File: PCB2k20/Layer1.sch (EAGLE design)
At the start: 279 parts, among them J1 XT30PB-F, J10 14AWG, J11 14AWG, J13 14AWG, J14 14AWG, J15 14AWG, J16 14AWG, J17 14AWG, J18 14AWG, J19 14AWG, J20 14AWG, J3 14AWG, J4 14AWG, J5 14AWG, J6 14AWG, J7 14AWG, J8 14AWG, J9 14AWG, Q1M1 AOD482, Q1M2 AOD482, Q1M3 AOD482, Q1M4 AOD482, U1M1 VNH5019, U1M2 VNH5019, U1M3 VNH5019, U1M4 VNH5019, X1 BM10B-SRSS-TB

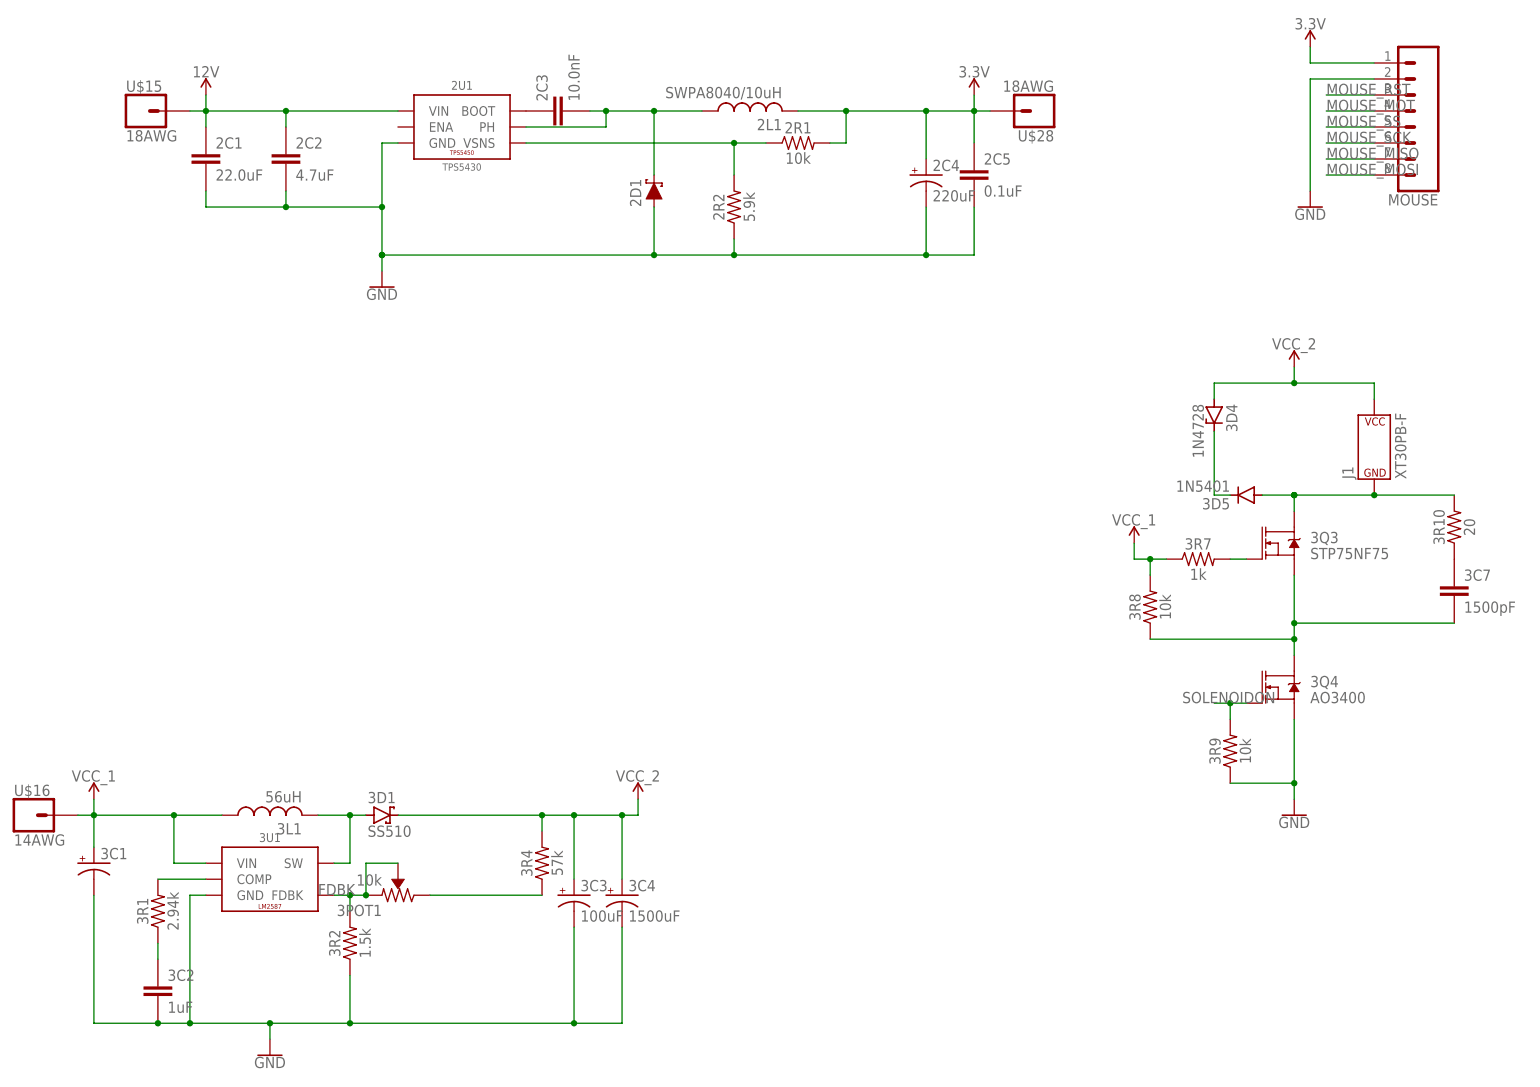
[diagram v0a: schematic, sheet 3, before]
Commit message: add gerbers, please everything turn out well!
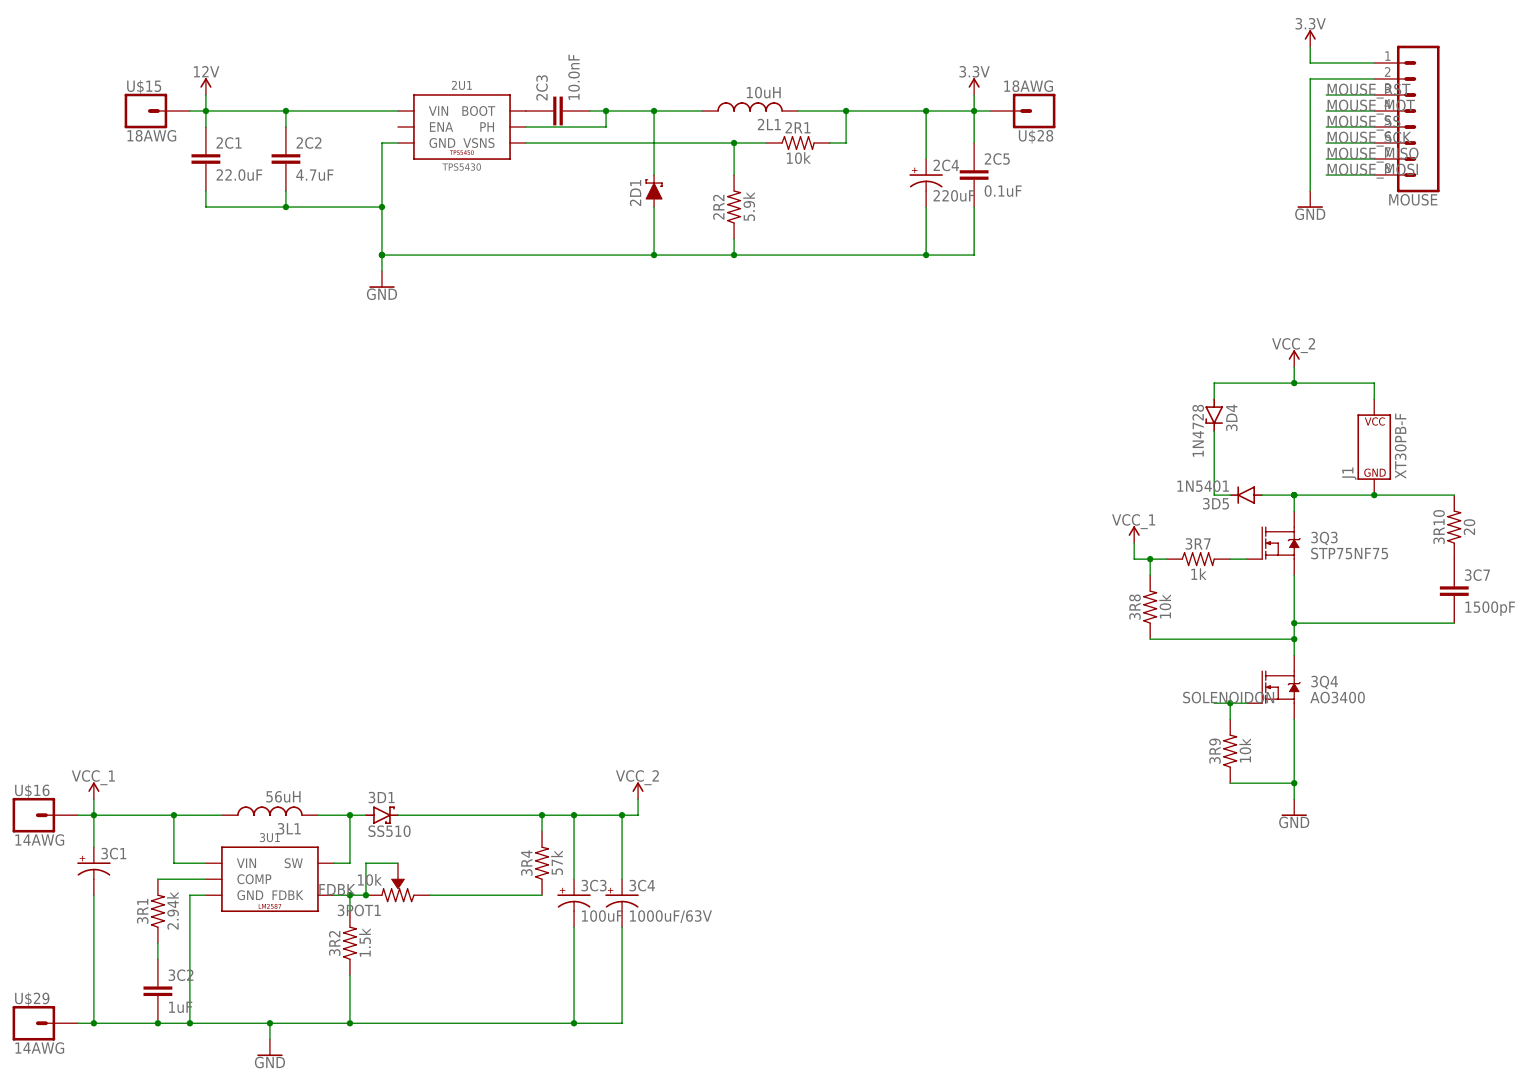
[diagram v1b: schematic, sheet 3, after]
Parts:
- added J21, U$29: 14AWG, JH:14AWG
- 2L1: value SWPA8040/10uH -> 10uH
- 3C4: value 1500uF -> 1000uF/63V
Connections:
- net GND: now also J21.1, U$29.1
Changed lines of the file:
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@@
 <part name="2C3" library="JH" library_urn="urn:adsk.eagle:library:6027132" deviceset="CAPACITOR" device="0603" package3d_urn="urn:adsk.eagle:package:15441226/3" value="10.0nF"/>
 <part name="2D1" library="SparkFun-DiscreteSemi" library_urn="urn:adsk.eagle:library:514" deviceset="DIODE-SCHOTTKY" device="-B340A" package3d_urn="urn:adsk.eagle:package:38443/1" value="3A/40V/500mV"/>
-<part name="2L1" library="JH" library_urn="urn:adsk.eagle:library:6027132" deviceset="INDUCTOR" device="SWPA8040" package3d_urn="urn:adsk.eagle:package:15402033/4" value="SWPA8040/10uH"/>
+<part name="2L1" library="JH" library_urn="urn:adsk.eagle:library:6027132" deviceset="INDUCTOR" device="SWPA8040" package3d_urn="urn:adsk.eagle:package:15402033/4" value="10uH"/>
 <part name="2R1" library="JH" library_urn="urn:adsk.eagle:library:6027132" deviceset="RESISTOR" device="0603" package3d_urn="urn:adsk.eagle:package:15441228/3" value="10k"/>
 <part name="2C4" library="rcl" library_urn="urn:adsk.eagle:library:334" deviceset="CPOL-US" device="D/7343-31R" package3d_urn="urn:adsk.eagle:package:23417/2" value="220uF"/>
@@
 <part name="SUPPLY25" library="SparkFun-PowerSymbols" library_urn="urn:adsk.eagle:library:530" deviceset="12V" device=""/>
 <part name="SUPPLY26" library="SparkFun-PowerSymbols" library_urn="urn:adsk.eagle:library:530" deviceset="3.3V" device=""/>
-<part name="CONN_M1" library="JH" library_urn="urn:adsk.eagle:library:6027132" deviceset="XT30" device="PB-F" package3d_urn="urn:adsk.eagle:package:15925142/4"/>
+<part name="CONN_M1" library="JH" library_urn="urn:adsk.eagle:library:6027132" deviceset="XT30" device="PB-F" package3d_urn="urn:adsk.eagle:package:15925142/7"/>
 <part name="U$4" library="JH" library_urn="urn:adsk.eagle:library:6027132" deviceset="74LVC2G" device="" package3d_urn="urn:adsk.eagle:package:16673544/1"/>
 <part name="U$5" library="JH" library_urn="urn:adsk.eagle:library:6027132" deviceset="74LVC2G" device="" package3d_urn="urn:adsk.eagle:package:16673544/1"/>
@@
 <part name="D2M2" library="SparkFun-LED" library_urn="urn:adsk.eagle:library:529" deviceset="LED-RED" device="0603" package3d_urn="urn:adsk.eagle:package:39354/1" value="RED"/>
 <part name="R12M2" library="JH" library_urn="urn:adsk.eagle:library:6027132" deviceset="RESISTOR" device="0603" package3d_urn="urn:adsk.eagle:package:15441228/3" value="4.7k"/>
-<part name="CONN_M2" library="JH" library_urn="urn:adsk.eagle:library:6027132" deviceset="XT30" device="PB-F" package3d_urn="urn:adsk.eagle:package:15925142/4"/>
+<part name="CONN_M2" library="JH" library_urn="urn:adsk.eagle:library:6027132" deviceset="XT30" device="PB-F" package3d_urn="urn:adsk.eagle:package:15925142/7"/>
 <part name="D1M3" library="SparkFun-LED" library_urn="urn:adsk.eagle:library:529" deviceset="LED-GREEN" device="0603" package3d_urn="urn:adsk.eagle:package:39354/1" value="GREEN"/>
 <part name="D2M3" library="SparkFun-LED" library_urn="urn:adsk.eagle:library:529" deviceset="LED-RED" device="0603" package3d_urn="urn:adsk.eagle:package:39354/1" value="RED"/>
 <part name="R12M3" library="JH" library_urn="urn:adsk.eagle:library:6027132" deviceset="RESISTOR" device="0603" package3d_urn="urn:adsk.eagle:package:15441228/3" value="4.7k"/>
-<part name="CONN_M3" library="JH" library_urn="urn:adsk.eagle:library:6027132" deviceset="XT30" device="PB-F" package3d_urn="urn:adsk.eagle:package:15925142/4"/>
+<part name="CONN_M3" library="JH" library_urn="urn:adsk.eagle:library:6027132" deviceset="XT30" device="PB-F" package3d_urn="urn:adsk.eagle:package:15925142/7"/>
 <part name="D1M4" library="SparkFun-LED" library_urn="urn:adsk.eagle:library:529" deviceset="LED-GREEN" device="0603" package3d_urn="urn:adsk.eagle:package:39354/1" value="GREEN"/>
 <part name="D2M4" library="SparkFun-LED" library_urn="urn:adsk.eagle:library:529" deviceset="LED-RED" device="0603" package3d_urn="urn:adsk.eagle:package:39354/1" value="RED"/>
 <part name="R12M4" library="JH" library_urn="urn:adsk.eagle:library:6027132" deviceset="RESISTOR" device="0603" package3d_urn="urn:adsk.eagle:package:15441228/3" value="4.7k"/>
-<part name="CONN_M4" library="JH" library_urn="urn:adsk.eagle:library:6027132" deviceset="XT30" device="PB-F" package3d_urn="urn:adsk.eagle:package:15925142/4"/>
+<part name="CONN_M4" library="JH" library_urn="urn:adsk.eagle:library:6027132" deviceset="XT30" device="PB-F" package3d_urn="urn:adsk.eagle:package:15925142/7"/>
 <part name="GND24" library="SparkFun-PowerSymbols" library_urn="urn:adsk.eagle:library:530" deviceset="GND" device=""/>
 <part name="SUPPLY29" library="SparkFun-PowerSymbols" library_urn="urn:adsk.eagle:library:530" deviceset="VCC_2" device=""/>
@@
 <part name="SUPPLY31" library="SparkFun-PowerSymbols" deviceset="3.3V" device=""/>
 <part name="GND26" library="SparkFun-PowerSymbols" library_urn="urn:adsk.eagle:library:530" deviceset="GND" device=""/>
-<part name="3C4" library="JH" library_urn="urn:adsk.eagle:library:6027132" deviceset="1000UF-CAP" device="" package3d_urn="urn:adsk.eagle:package:7103959/4" value="1500uF"/>
+<part name="3C4" library="JH" library_urn="urn:adsk.eagle:library:6027132" deviceset="1000UF-CAP" device="" package3d_urn="urn:adsk.eagle:package:7103959/4" value="1000uF/63V"/>
 <part name="1PT37" library="SparkFun-Sensors" deviceset="LIGHT_SENSOR" device="ALS"/>
 <part name="1PT38" library="SparkFun-Sensors" deviceset="LIGHT_SENSOR" device="ALS"/>
@@
 <part name="3C7" library="JH" library_urn="urn:adsk.eagle:library:6027132" deviceset="CAPACITOR" device="0603" package3d_urn="urn:adsk.eagle:package:15441226/3" value="1500pF"/>
 <part name="3R10" library="JH" library_urn="urn:adsk.eagle:library:6027132" deviceset="RESISTOR" device="0603" package3d_urn="urn:adsk.eagle:package:15441228/3" value="20"/>
-<part name="J1" library="JH" library_urn="urn:adsk.eagle:library:6027132" deviceset="XT30" device="PB-F" package3d_urn="urn:adsk.eagle:package:15925142/4"/>
+<part name="J1" library="JH" library_urn="urn:adsk.eagle:library:6027132" deviceset="XT30" device="PB-F" package3d_urn="urn:adsk.eagle:package:15925142/7"/>
 <part name="U$6" library="SparkFun-PowerSymbols" library_urn="urn:adsk.eagle:library:530" deviceset="VCCA" device=""/>
 <part name="U$7" library="SparkFun-PowerSymbols" library_urn="urn:adsk.eagle:library:530" deviceset="VCCA" device=""/>
@@
 <part name="U$27" library="JH" library_urn="urn:adsk.eagle:library:6027132" deviceset="18AWG" device="" package3d_urn="urn:adsk.eagle:package:16754415/1"/>
 <part name="U$28" library="JH" library_urn="urn:adsk.eagle:library:6027132" deviceset="18AWG" device="" package3d_urn="urn:adsk.eagle:package:16754415/1"/>
+<part name="U$29" library="JH" library_urn="urn:adsk.eagle:library:6027132" deviceset="14AWG" device="" package3d_urn="urn:adsk.eagle:package:16673531/1"/>
+<part name="J21" library="JH" library_urn="urn:adsk.eagle:library:6027132" deviceset="14AWG" device="" package3d_urn="urn:adsk.eagle:package:16673531/1"/>
 </parts>
 <sheets>
@@
 <attribute name="NAME" x="180.34" y="156.972" size="1.778" layer="95" font="vector" rot="R180"/>
 </instance>
+<instance part="U$29" gate="G$1" x="17.78" y="15.24" smashed="yes">
+<attribute name="VALUE" x="15.24" y="10.414" size="1.778" layer="96" font="vector"/>
+<attribute name="NAME" x="15.24" y="18.288" size="1.778" layer="95" font="vector"/>
+</instance>
 </instances>
 <busses>
@@
 <wire x1="111.76" y1="15.24" x2="104.14" y2="15.24" width="0.1524" layer="91"/>
 <junction x="104.14" y="15.24"/>
+<pinref part="U$29" gate="G$1" pin="1"/>
+<wire x1="25.4" y1="15.24" x2="27.94" y2="15.24" width="0.1524" layer="91"/>
+<junction x="27.94" y="15.24"/>
 </segment>
 <segment>
@@
 <attribute name="VALUE" x="160.02" y="86.106" size="1.778" layer="96" align="top-center"/>
 </instance>
+<instance part="J21" gate="G$1" x="124.46" y="139.7" smashed="yes">
+<attribute name="VALUE" x="121.92" y="134.874" size="1.778" layer="96" font="vector"/>
+<attribute name="NAME" x="121.92" y="142.748" size="1.778" layer="95" font="vector"/>
+</instance>
 </instances>
 <busses>
@@
 <wire x1="134.62" y1="66.04" x2="134.62" y2="78.74" width="0.1524" layer="91"/>
 <wire x1="104.14" y1="142.24" x2="134.62" y2="142.24" width="0.1524" layer="91"/>
-<wire x1="134.62" y1="142.24" x2="134.62" y2="129.54" width="0.1524" layer="91"/>
+<wire x1="134.62" y1="142.24" x2="134.62" y2="139.7" width="0.1524" layer="91"/>
 <pinref part="J6" gate="G$1" pin="1"/>
+<wire x1="134.62" y1="139.7" x2="134.62" y2="129.54" width="0.1524" layer="91"/>
 <wire x1="134.62" y1="129.54" x2="134.62" y2="116.84" width="0.1524" layer="91"/>
 <wire x1="132.08" y1="129.54" x2="134.62" y2="129.54" width="0.1524" layer="91"/>
@@
 <wire x1="132.08" y1="66.04" x2="134.62" y2="66.04" width="0.1524" layer="91"/>
 <junction x="134.62" y="66.04"/>
+<pinref part="J21" gate="G$1" pin="1"/>
+<wire x1="132.08" y1="139.7" x2="134.62" y2="139.7" width="0.1524" layer="91"/>
+<junction x="134.62" y="139.7"/>
 </segment>
 <segment>
